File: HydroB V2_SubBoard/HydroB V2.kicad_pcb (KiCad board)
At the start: 4 copper layers, 109.5 x 82.5 mm, 78 parts, among them J1 Conn_01x02_Pin, J10 Screw_Terminal_01x02, J16 Screw_Terminal_01x02, J2 Conn_01x02_Pin, J3 Screw_Terminal_01x02, J4 Conn_01x04_Pin, J5 PH SENSOR, J6 EC SENSOR, J7 Conn_01x02_Pin, J8 Screw_Terminal_01x02, J9 Screw_Terminal_01x02, Q1 S8050, Q2 S8050, Q3 S8050, Q4 S8050, Q8 S8050, SW1 SW_Push, U1 STM32F103C8Tx, U3 SN65HVD72DR, U4 LMR33620ADDA, U5 SN65HVD230, Y1 8Mhz

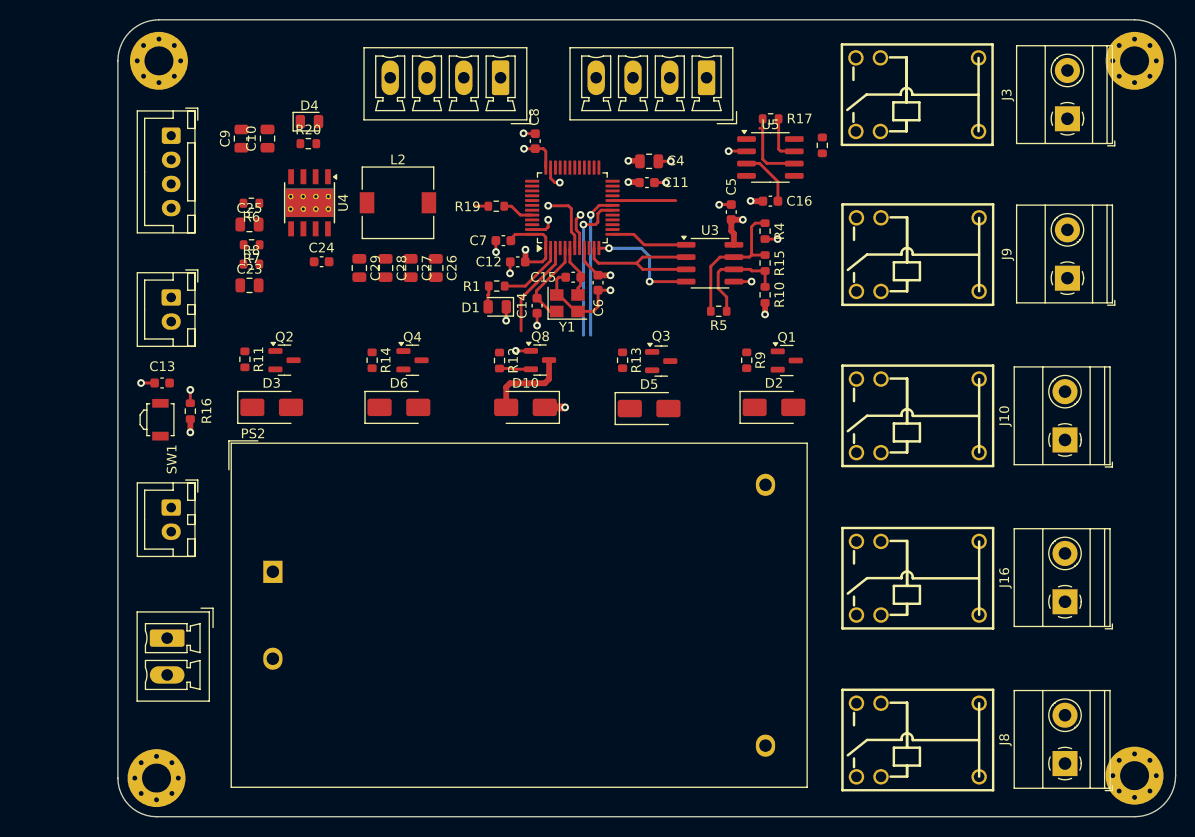
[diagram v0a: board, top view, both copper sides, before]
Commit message: PCB layout update
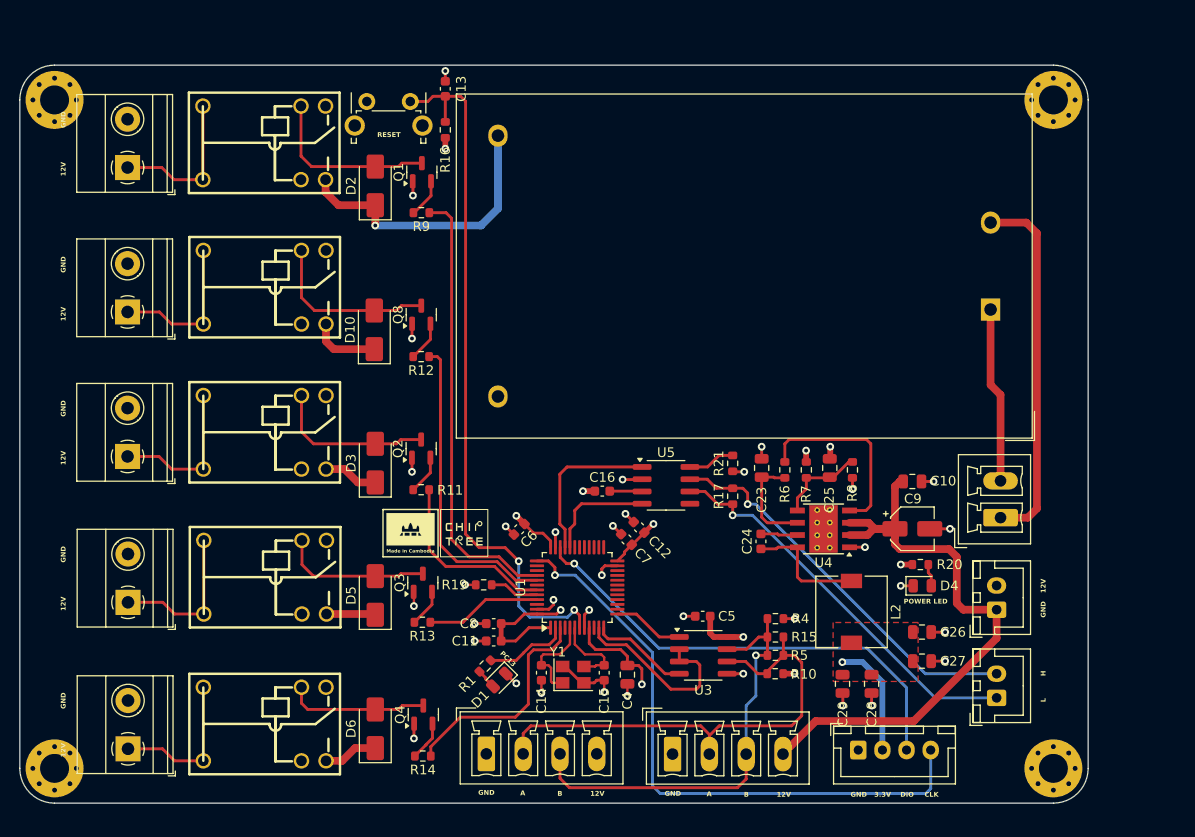
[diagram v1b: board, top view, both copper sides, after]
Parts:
- added G***: LOGO, CHIPTREE_LOGO:cam5x5, F.Cu at (123.0, 108.2)
- added G***: LOGO, CHIPTREE_LOGO:CHPTREE-5x5mm, F.Cu at (128.6, 108.7)
- C9: footprint Capacitor_SMD:C_0805_2012Metric -> Capacitor_SMD:CP_Elec_4x3
- SW1: footprint Button_Switch_SMD:SW_SPST_B3U-3000P -> Button_Switch_THT:SW_Tactile_SPST_Angled_PTS645Vx39-2LFS
- moved H5 111.9 mm to (86.2, 63.8)
- moved H6 111.8 mm to (86.2, 133.0)
- moved J9 102.9 mm to (93.8, 115.8)
- moved J10 102.1 mm to (93.8, 131.0)
- moved J8 102.1 mm to (93.8, 100.7)
- moved J16 101.6 mm to (93.8, 85.8)
- moved J3 97.4 mm to (93.8, 70.8)
- moved J4 95.4 mm to (169.4, 131.1), turned to 0 degrees
- moved J1 95.0 mm to (183.7, 125.7), turned to 90 degrees
- moved H8 92.9 mm to (189.6, 133.0)
- moved H7 92.7 mm to (189.6, 63.8)
- moved J7 87.2 mm to (184.1, 107.0), turned to 90 degrees
- moved J2 86.1 mm to (183.7, 116.6), turned to 90 degrees
- moved C9 80.4 mm to (175.0, 108.2), turned to 0 degrees
- moved D4 79.6 mm to (176.0, 114.1)
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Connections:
- U1 pad 18: /HydroB/Block Relay1/RELAY_2 -> unconnected-(U1-PB0-Pad18)
- U1 pad 19: /HydroB/Block Relay1/RELAY_4 -> unconnected-(U1-PB1-Pad19)
- U1 pad 20: /HydroB/Block Relay1/RELAY_1 -> unconnected-(U1-PB2-Pad20)
- U1 pad 40: unconnected-(U1-PB4-Pad40) -> /HydroB/Block Relay1/RELAY_1
- U1 pad 41: unconnected-(U1-PB5-Pad41) -> /HydroB/Block Relay1/RELAY_2
- U1 pad 43: unconnected-(U1-PB7-Pad43) -> /HydroB/Block Relay1/RELAY_3
- U1 pad 45: unconnected-(U1-PB8-Pad45) -> /HydroB/Block Relay1/RELAY_4
- U1 pad 46: /HydroB/Block Relay1/RELAY_3 -> unconnected-(U1-PB9-Pad46)
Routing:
- net +12V: track 2.10 -> 117.0 mm
- net NRST: track 8.19 -> 73.6 mm
- net SWCLK: track 0.00 -> 63.5 mm, vias 0 -> 1
- net SWDIO: track 0.00 -> 48.9 mm, vias 0 -> 1
- net Net-(J5-Pin_2): track 11.1 -> 53.3 mm
- net /HydroB/Block Relay1/RELAY_1: track 6.55 -> 46.2 mm
- net N: track 0.00 -> 37.9 mm
- net Net-(J1-Pin_2): track 4.84 -> 40.8 mm, vias 0 -> 1
- net Net-(J1-Pin_1): track 7.64 -> 41.3 mm, vias 0 -> 1
- net +3.3V: track 28.8 -> 59.9 mm, vias 9 -> 12
- net Net-(J5-Pin_3): track 15.2 -> 45.5 mm, vias 0 -> 1
- net PG: track 0.00 -> 20.0 mm
- net /HydroB/Block Relay1/RELAY_3: track 0.00 -> 19.1 mm
- net Net-(D2-A): track 0.00 -> 18.3 mm
- net L: track 0.00 -> 18.2 mm
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- added copper zone on In2.Cu, net +12V
- added copper zone on F.Cu, net +3.3V
- added copper zone on In2.Cu, net +3.3V
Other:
- board size 109.5 x 82.5 mm -> 110.6 x 76.4 mm
- board text added: "12V"
- board text added: "3.3V"
- board text added: "A"
- board text added: "B"
- board text added: "CLK"
- board text added: "DIO"
- board text added: "GND"
- board text added: "H"
- board text added: "L"
- board text added: "Made in Cambodia"
- board text added: "PC13"
- board text added: "POWER LED"
- board text added: "RESET"
